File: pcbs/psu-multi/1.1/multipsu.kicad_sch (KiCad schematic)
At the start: 56 parts, among them J1 Conn_01x06_Pin, J2 Conn_01x03_Male, J3 Conn_01x02_Pin, J4 Conn_01x03_Pin, J5 Conn_01x03_Pin, J6 Conn_01x02_Pin, J7 Conn_01x03_Pin, U1 LM337_SOT223, U2 LM317_SOT-223, U3 ZLDO1117QG33TA, U4 AMS1117-5.0, U5 NCP1117-12, U6 TMP100, U7 AP64351SP-13

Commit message: UPdates
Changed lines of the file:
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@@
 (kicad_sch
-	(version 20231120)
+	(version 20250114)
 	(generator "eeschema")
-	(generator_version "8.0")
+	(generator_version "9.0")
 	(paper "A2")
 	(junction
@@
 		)
 	)
+	(embedded_fonts no)
 )

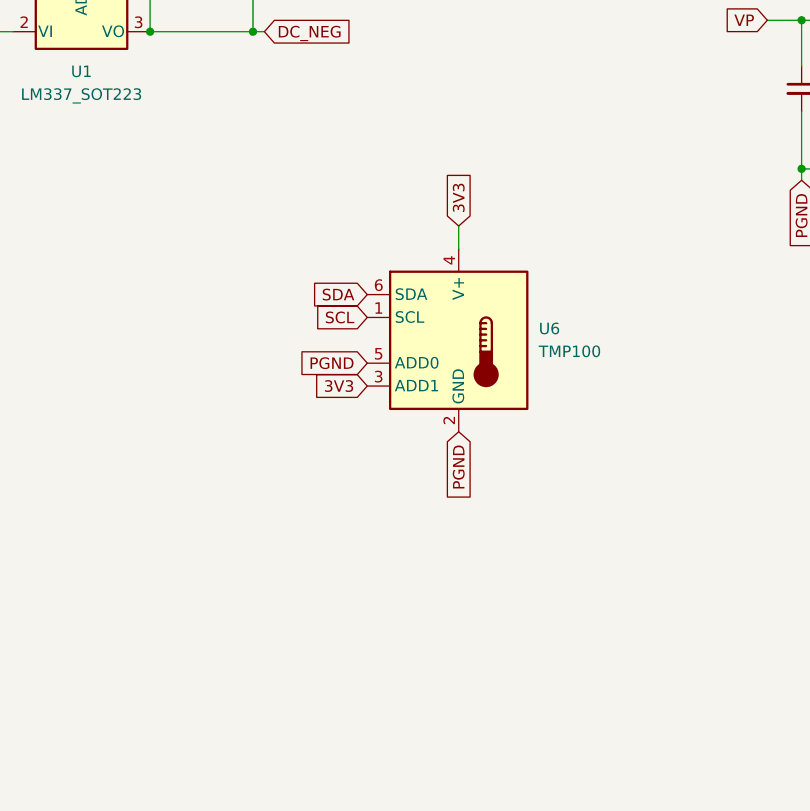
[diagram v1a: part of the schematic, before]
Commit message: Updates
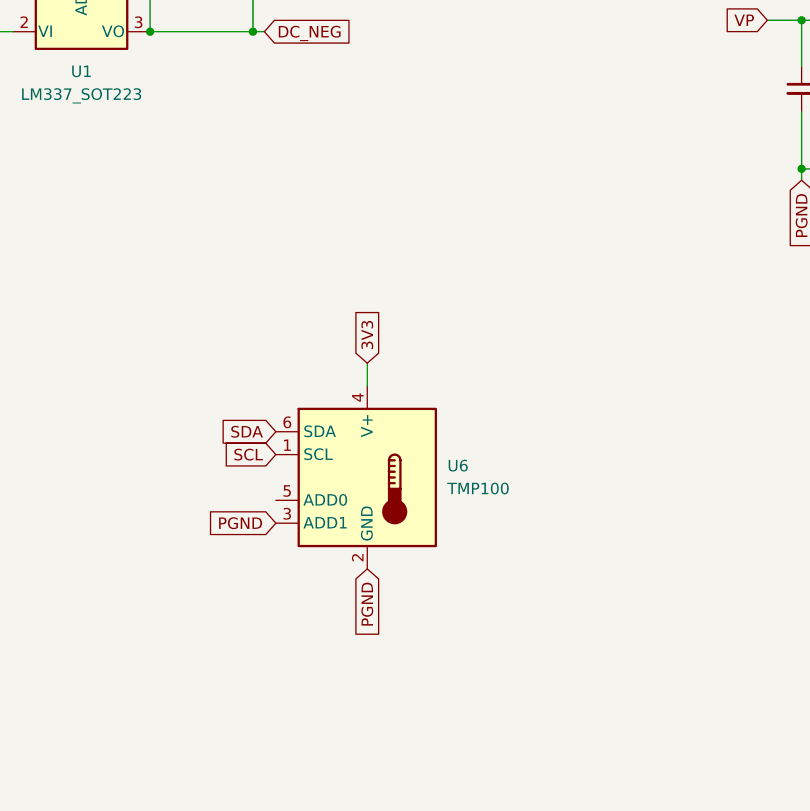
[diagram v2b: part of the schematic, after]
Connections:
- net 3V3: no longer U6.3 (ADD1)
- net PGND: now also U6.3 (ADD1); no longer U6.5 (ADD0)
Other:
- moved on the sheet: U6
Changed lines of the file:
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@@
 	(wire
 		(pts
-			(xy 118.11 156.21) (xy 118.11 158.75)
+			(xy 107.95 171.45) (xy 107.95 173.99)
 		)
 		(stroke
@@
 	(global_label "3V3"
 		(shape input)
-		(at 118.11 156.21 90)
+		(at 107.95 171.45 90)
 		(fields_autoplaced yes)
 		(effects
@@
 		)
 		(property "Intersheetrefs" "${INTERSHEET_REFS}"
-			(at 118.11 149.7172 90)
+			(at 107.95 164.9572 90)
 			(effects
 				(font
@@
 	(global_label "SDA"
 		(shape input)
-		(at 107.95 163.83 180)
+		(at 97.79 179.07 180)
 		(fields_autoplaced yes)
 		(effects
@@
 		)
 		(property "Intersheetrefs" "${INTERSHEET_REFS}"
-			(at 101.3967 163.83 0)
+			(at 91.2367 179.07 0)
 			(effects
 				(font
@@
 	(global_label "SCL"
 		(shape input)
-		(at 107.95 166.37 180)
+		(at 97.79 181.61 180)
 		(fields_autoplaced yes)
 		(effects
@@
 		)
 		(property "Intersheetrefs" "${INTERSHEET_REFS}"
-			(at 101.4572 166.37 0)
+			(at 91.2972 181.61 0)
 			(effects
 				(font
@@
 		)
 	)
-	(global_label "3V3"
+	(global_label "RELAY_GND"
 		(shape input)
-		(at 107.95 173.99 180)
+		(at 68.58 63.5 0)
 		(fields_autoplaced yes)
 		(effects
@@
 				(size 1.27 1.27)
 			)
-			(justify right)
+			(justify left)
 		)
 		(property "Intersheetrefs" "${INTERSHEET_REFS}"
-			(at 101.4572 173.99 0)
+			(at 82.0276 63.5 0)
 			(effects
 				(font
 					(size 1.27 1.27)
 				)
-				(justify right)
+				(justify left)
 				(hide yes)
 			)
 		)
 	)
-	(global_label "RELAY_GND"
+	(global_label "GND"
 		(shape input)
-		(at 68.58 63.5 0)
+		(at 248.92 148.59 270)
 		(fields_autoplaced yes)
 		(effects
@@
 				(size 1.27 1.27)
 			)
-			(justify left)
+			(justify right)
 		)
 		(property "Intersheetrefs" "${INTERSHEET_REFS}"
-			(at 82.0276 63.5 0)
+			(at 248.92 155.4457 90)
 			(effects
 				(font
 					(size 1.27 1.27)
 				)
-				(justify left)
+				(justify right)
 				(hide yes)
 			)
 		)
 	)
-	(global_label "GND"
+	(global_label "AGND"
 		(shape input)
-		(at 248.92 148.59 270)
+		(at 74.93 294.64 0)
 		(fields_autoplaced yes)
 		(effects
@@
 				(size 1.27 1.27)
 			)
-			(justify right)
+			(justify left)
 		)
 		(property "Intersheetrefs" "${INTERSHEET_REFS}"
-			(at 248.92 155.4457 90)
+			(at 82.8743 294.64 0)
 			(effects
 				(font
 					(size 1.27 1.27)
 				)
-				(justify right)
+				(justify left)
 				(hide yes)
 			)
 		)
 	)
-	(global_label "AGND"
+	(global_label "PGND"
 		(shape input)
-		(at 74.93 294.64 0)
+		(at 97.79 189.23 180)
 		(fields_autoplaced yes)
 		(effects
@@
 				(size 1.27 1.27)
 			)
-			(justify left)
+			(justify right)
 		)
 		(property "Intersheetrefs" "${INTERSHEET_REFS}"
-			(at 82.8743 294.64 0)
+			(at 89.6643 189.23 0)
 			(effects
 				(font
 					(size 1.27 1.27)
 				)
-				(justify left)
+				(justify right)
 				(hide yes)
 			)
@@
 	(global_label "PGND"
 		(shape input)
-		(at 118.11 179.07 270)
+		(at 107.95 194.31 270)
 		(fields_autoplaced yes)
 		(effects
@@
 		)
 		(property "Intersheetrefs" "${INTERSHEET_REFS}"
-			(at 118.11 187.1957 90)
+			(at 107.95 202.4357 90)
 			(effects
 				(font
@@
 		)
 	)
-	(global_label "PGND"
-		(shape input)
-		(at 107.95 171.45 180)
-		(fields_autoplaced yes)
-		(effects
-			(font
-				(size 1.27 1.27)
-			)
-			(justify right)
-		)
-		(property "Intersheetrefs" "${INTERSHEET_REFS}"
-			(at 99.8243 171.45 0)
-			(effects
-				(font
-					(size 1.27 1.27)
-				)
-				(justify right)
-				(hide yes)
-			)
-		)
-	)
 	(global_label "3V3"
 		(shape input)
@@
 	(symbol
 		(lib_id "Sensor_Temperature:TMP100")
-		(at 118.11 168.91 0)
+		(at 107.95 184.15 0)
 		(unit 1)
 		(exclude_from_sim no)
@@
 		(fields_autoplaced yes)
 		(property "Reference" "U6"
-			(at 127 167.6399 0)
+			(at 116.84 182.8799 0)
 			(effects
 				(font
@@
 		)
 		(property "Value" "TMP100"
-			(at 127 170.1799 0)
+			(at 116.84 185.4199 0)
 			(effects
 				(font
@@
 		)
 		(property "Footprint" "Package_TO_SOT_SMD:SOT-23-6"
-			(at 118.11 177.8 0)
+			(at 107.95 193.04 0)
 			(effects
 				(font
@@
 		)
 		(property "Datasheet" "http://www.ti.com/lit/gpn/tmp100"
-			(at 116.84 168.91 0)
+			(at 106.68 184.15 0)
 			(effects
 				(font
@@
 		)
 		(property "Description" "Temperature Sensor with I2C/SMBus Interface, SOT-23-6"
-			(at 118.11 168.91 0)
+			(at 107.95 184.15 0)
 			(effects
 				(font
